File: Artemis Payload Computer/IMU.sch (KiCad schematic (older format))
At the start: 1 part, among them U401 ICM-20948

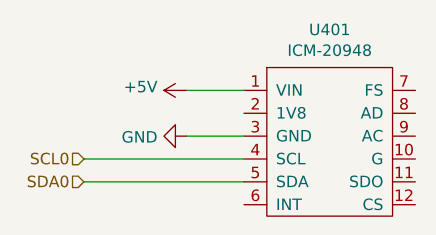
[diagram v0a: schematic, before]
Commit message: big commit, sorry. sd card needs finishing
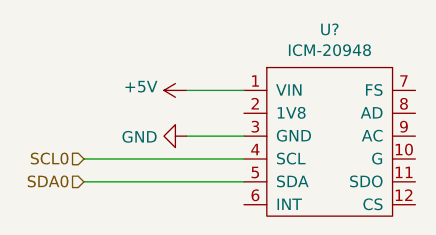
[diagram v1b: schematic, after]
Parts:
- renumbered U401 to U?
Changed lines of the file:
@@
 $Descr A4 11693 8268
 encoding utf-8
-Sheet 4 6
+Sheet 4 7
 Title ""
 Date ""
@@
 $EndDescr
 $Comp
-L Artemis_Footprints:ICM-20948 U401
+L Artemis_Footprints:ICM-20948 U?
 U 1 1 60405DA7
 P 6200 3000
-F 0 "U401" H 6225 3165 50  0000 C CNN
+F 0 "U?" H 6225 3165 50  0000 C CNN
 F 1 "ICM-20948" H 6225 3074 50  0000 C CNN
 F 2 "Artemis Payload Computer:ICM-20948" H 6200 3000 50  0001 C CNN
@@
 $EndComp
 $Comp
-L power:+5V #PWR0109
+L power:+5V #PWR?
 U 1 1 604076E6
 P 5600 3100
-F 0 "#PWR0109" H 5600 2950 50  0001 C CNN
+F 0 "#PWR?" H 5600 2950 50  0001 C CNN
 F 1 "+5V" V 5615 3228 50  0000 L CNN
 F 2 "" H 5600 3100 50  0001 C CNN
@@
 $EndComp
 $Comp
-L power:GND #PWR0110
+L power:GND #PWR?
 U 1 1 604079B0
 P 5600 3300
-F 0 "#PWR0110" H 5600 3050 50  0001 C CNN
+F 0 "#PWR?" H 5600 3050 50  0001 C CNN
 F 1 "GND" V 5605 3172 50  0000 R CNN
 F 2 "" H 5600 3300 50  0001 C CNN
